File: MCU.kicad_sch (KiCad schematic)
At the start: 26 parts, among them J3 ST_LINK, SW1 Reset, U1 STM32G070CBT6, U5 LM4040DBZ-3, Y1 FC-135R_32.7680KA-AG0

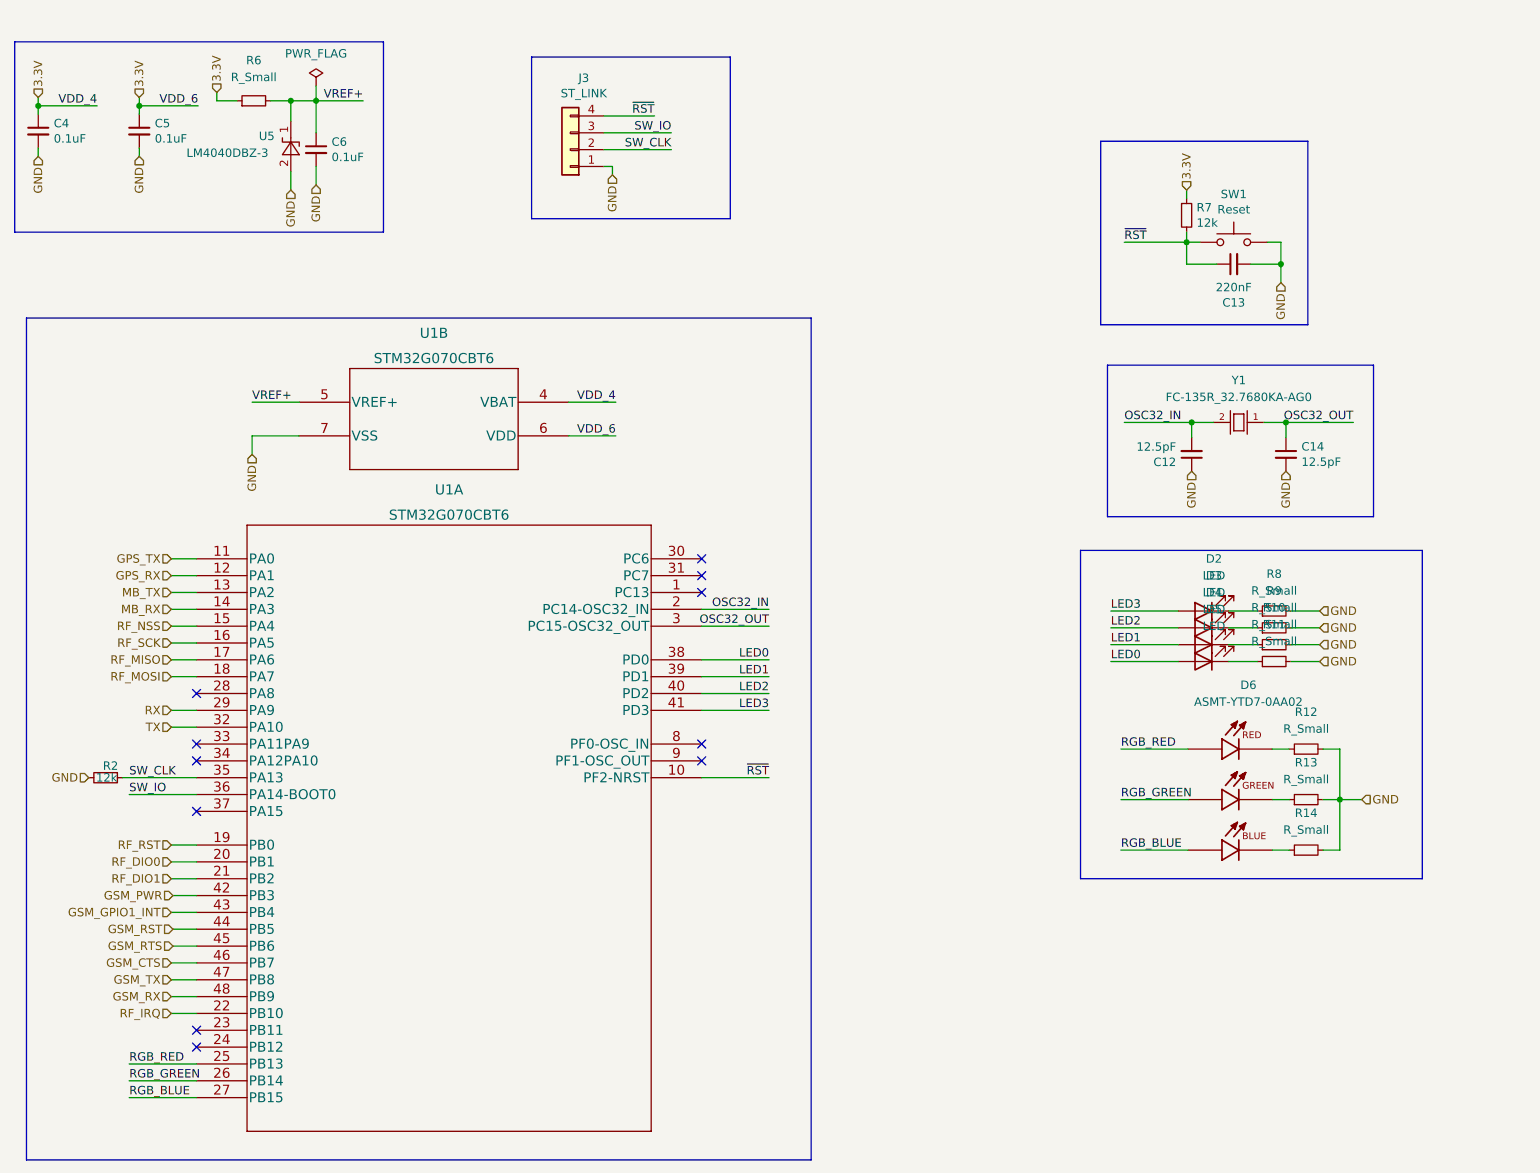
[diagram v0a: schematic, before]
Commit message: KiCad 0.2v
Schematics done.
Have to assign footprints to corresponding components.
Completely rework PCB.
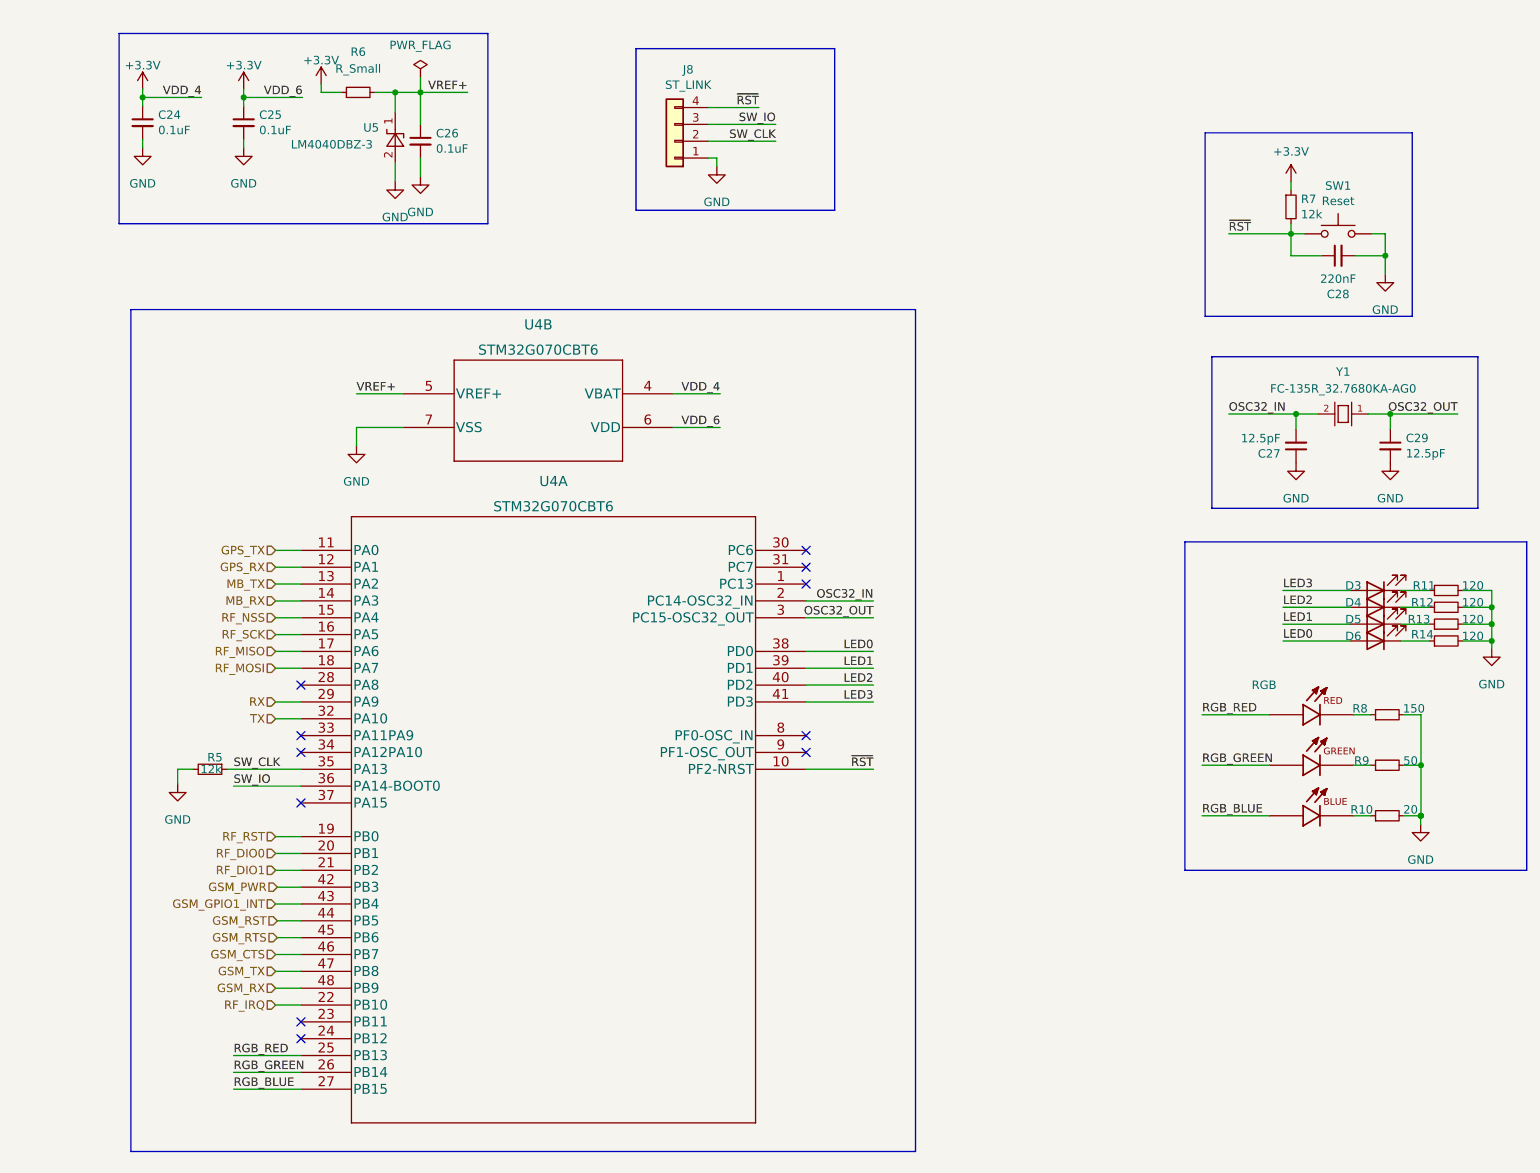
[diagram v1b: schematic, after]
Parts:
- removed C12, C14: 12.5pF, Capacitor_SMD:C_0603_1608Metric, symbol Device:C_Small
- removed C13: 220nF, Capacitor_SMD:C_0603_1608Metric, symbol Device:C_Small
- removed C4, C5, C6: 0.1uF, Capacitor_SMD:C_0603_1608Metric, symbol Device:C_Small
- removed D2: LED, symbol Device:LED
- removed D6: ASMT-YTD7-0AA02, LED_ASMT-YTD7-0AA02, symbol test:ASMT-YTD7-0AA02
- removed J3: ST_LINK, Connector_PinSocket_2.54mm:PinSocket_1x04_P2.54mm_Vertical, symbol Connector_Generic:Conn_01x04
- removed R2: 12k, Resistor_SMD:R_0603_1608Metric, symbol Device:R_Small
- removed U1: STM32G070CBT6, LQFP-48, symbol test:STM32G070CBT6
- added C24, C25, C26: 0.1uF, Capacitor_SMD:C_0603_1608Metric, symbol Device:C_Small
- added C27, C29: 12.5pF, Capacitor_SMD:C_0603_1608Metric, symbol Device:C_Small
- added C28: 220nF, Capacitor_SMD:C_0603_1608Metric, symbol Device:C_Small
- added D2: RGB, footprints:LED_ASMT-YTD7-0AA02, symbol test:ASMT-YTD7-0AA02
- added D6: LED, symbol Device:LED
- added J8: ST_LINK, Connector_PinSocket_2.54mm:PinSocket_1x04_P2.54mm_Vertical, symbol Connector_Generic:Conn_01x04
- added R5: 12k, Resistor_SMD:R_0603_1608Metric, symbol Device:R_Small
- added U4: STM32G070CBT6, LQFP-48, symbol test:STM32G070CBT6
- R10: value R_Small -> 20
- R11, R12, R13, R14: value R_Small -> 120
- R8: value R_Small -> 150
- R9: value R_Small -> 50
- Y1: footprint XTAL_FC-135R_32.7680KA-AG0 -> footprints:XTAL_FC-135R_32.7680KA-AG0
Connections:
- net GND: now also C24.2, C25.2, C26.2, C27.1, C28.2, C29.2, J8.1 (Pin_1), R5.2, U4.7 (VSS)
- net GPS_RX: now also U4.12 (PA1)
- net GPS_TX: now also U4.11 (PA0)
- net GSM_CTS: now also U4.46 (PB7)
- net GSM_GPIO1_INT: now also U4.43 (PB4)
- net GSM_PWR: now also U4.42 (PB3)
- net GSM_RST: now also U4.44 (PB5)
- net GSM_RTS: now also U4.45 (PB6)
- net GSM_RX: now also U4.48 (PB9)
- net GSM_TX: now also U4.47 (PB8)
- net LED0: now also D6.2 (A), U4.38 (PD0); no longer D5.2 (A)
- net LED1: now also D5.2 (A), U4.39 (PD1); no longer D4.2 (A)
- net LED2: now also D4.2 (A), U4.40 (PD2); no longer D3.2 (A)
- net LED3: now also D3.2 (A), U4.41 (PD3)
- net MB_RX: now also U4.14 (PA3)
- net MB_TX: now also U4.13 (PA2)
- net OSC32_IN: now also C27.2, U4.2 (PC14-OSC32_IN)
- net OSC32_OUT: now also C29.1, U4.3 (PC15-OSC32_OUT)
- net RF_DIO0: now also U4.20 (PB1)
- net RF_DIO1: now also U4.21 (PB2)
- net RF_IRQ: now also U4.22 (PB10)
- net RF_MISO: now also U4.17 (PA6)
- net RF_MOSI: now also U4.18 (PA7)
- net RF_NSS: now also U4.15 (PA4)
- net RF_RST: now also U4.19 (PB0)
- net RF_SCK: now also U4.16 (PA5)
- net RGB_BLUE: now also D2.6, U4.27 (PB15)
- net RGB_GREEN: now also D2.5, U4.26 (PB14)
- net RGB_RED: now also D2.4, U4.25 (PB13)
- net RX: now also U4.29 (PA9)
- net SW_CLK: now also J8.2 (Pin_2), R5.1, U4.35 (PA13)
- net SW_IO: now also J8.3 (Pin_3), U4.36 (PA14-BOOT0)
- net TX: now also U4.32 (PA10)
- net VREF+: now also C26.1, U4.5 (VREF+)
- net ~{RST}: now also C28.1, J8.4 (Pin_4), U4.10 (PF2-NRST)
- net at R13.1: now also D5.1 (K)
- net at R11.1: now also D3.1 (K); no longer D5.1 (K)
- net at R14.1: now also D6.1 (K)
- net at R9.1: now also D2.2; no longer D3.1 (K)
- net at R8.1: now also D2.3
- net at D4.1 (K): now also R12.1; no longer R10.1
- net 3.3V renamed +3V3
- net +3V3: now also C24.1, C25.1, U4.4 (VBAT), U4.6 (VDD)
- new net: D2.1, R10.1

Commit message: KiCad 0.3v
Improved aesthetics.
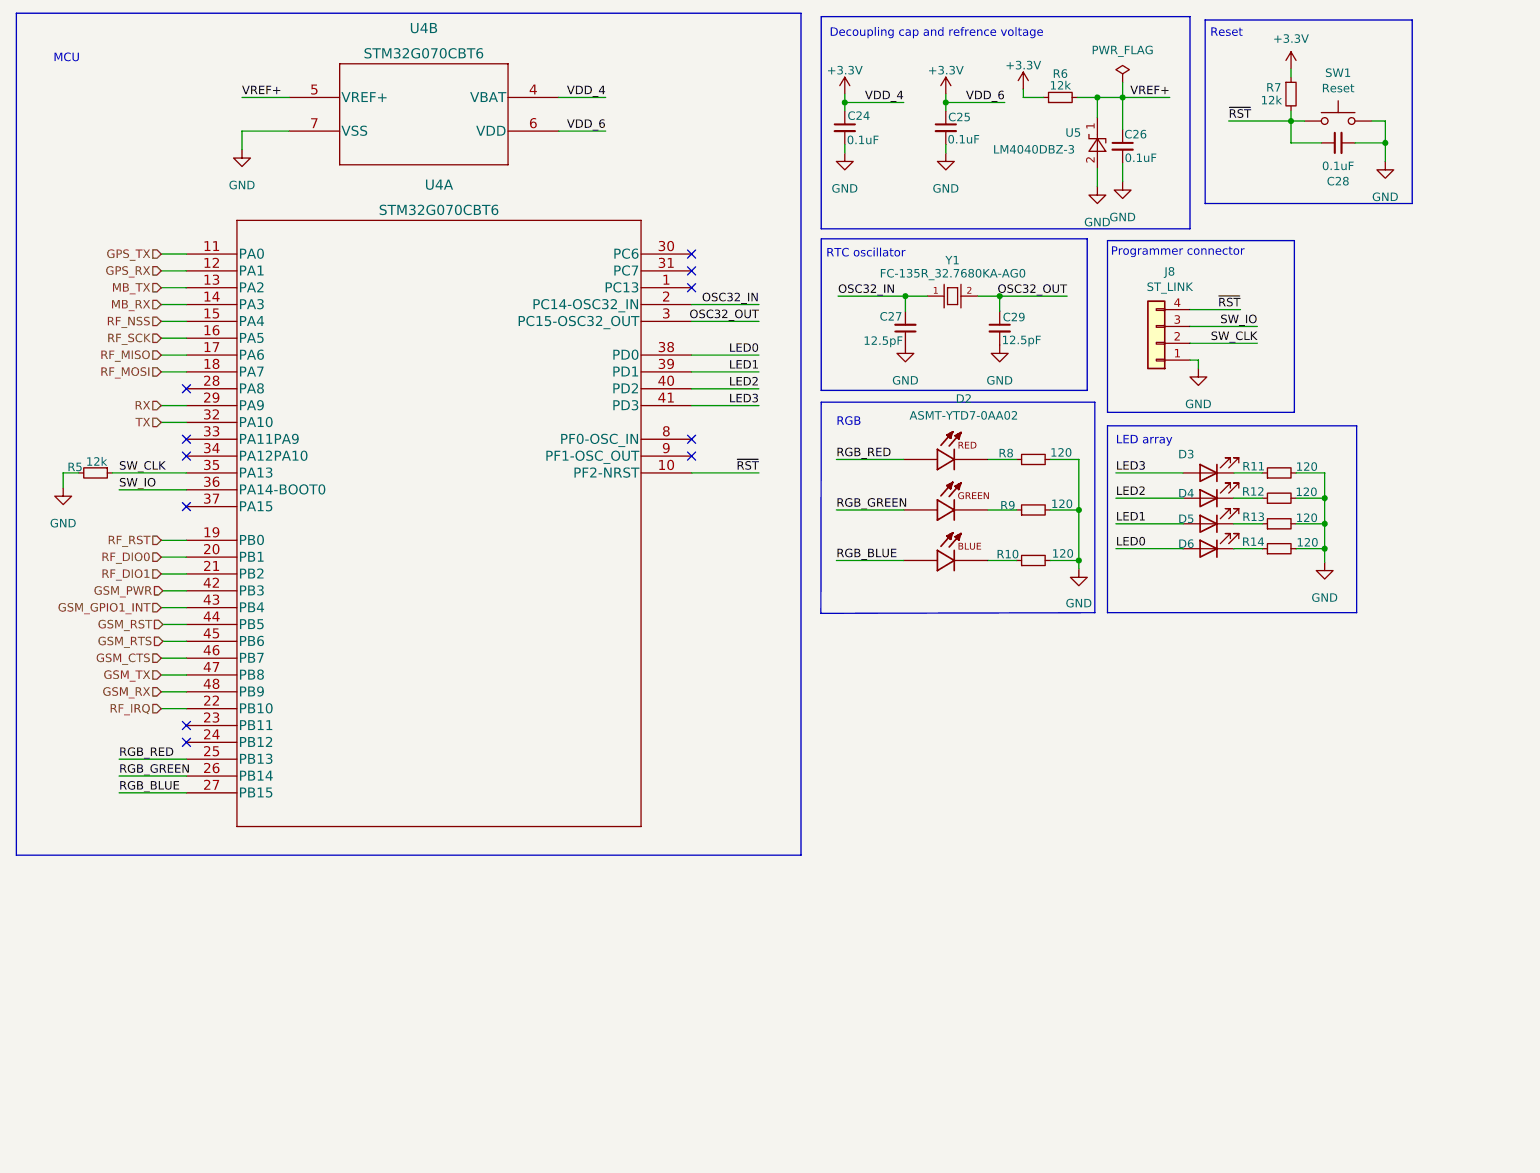
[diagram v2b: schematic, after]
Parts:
- removed D2: RGB, footprints:LED_ASMT-YTD7-0AA02, symbol test:ASMT-YTD7-0AA02
- removed Y1: FC-135R_32.7680KA-AG0, footprints:XTAL_FC-135R_32.7680KA-AG0, symbol test:FC-135R_32.7680KA-AG0
- added D2: ASMT-YTD7-0AA02, LED_ASMT-YTD7-0AA02, symbol schematics:ASMT-YTD7-0AA02
- added Y1: FC-135R_32.7680KA-AG0, XTAL_FC-135R_32.7680KA-AG0, symbol schematics:FC-135R_32.7680KA-AG0
- C28: value 220nF -> 0.1uF
- D3, D4, D5, D6: footprint (none) -> LED_SMD:LED_0603_1608Metric
- R10: value 20 -> 120; footprint (none) -> Resistor_SMD:R_0603_1608Metric
- R11, R12, R13, R14: footprint (none) -> Resistor_SMD:R_0603_1608Metric
- R6: value R_Small -> 12k; footprint (none) -> Resistor_SMD:R_0603_1608Metric
- R8: value 150 -> 120; footprint (none) -> Resistor_SMD:R_0603_1608Metric
- R9: value 50 -> 120; footprint (none) -> Resistor_SMD:R_0603_1608Metric
- U4: symbol test:STM32G070CBT6 -> schematics:STM32G070CBT6
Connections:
- net OSC32_IN: now also Y1.1
- net OSC32_OUT: now also Y1.2
- net RGB_BLUE: now also D2.6
- net RGB_GREEN: now also D2.5
- net RGB_RED: now also D2.4
- net at R9.1: now also D2.2
- net at R8.1: now also D2.3
- net at R10.1: now also D2.1
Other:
- note added: "Decoupling cap and refrence voltage"
- note added: "LED array"
- note added: "MCU"
- note added: "Programmer connector"
- note added: "RGB"
- note added: "RTC oscillator"
- note added: "Reset"
- moved on the sheet: C24, C25, C26, C27, C28, C29, D3, D4, D5, D6, J8, R10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

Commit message: 0.1v COM_PCB KiCad
First iteration of COM PCB.
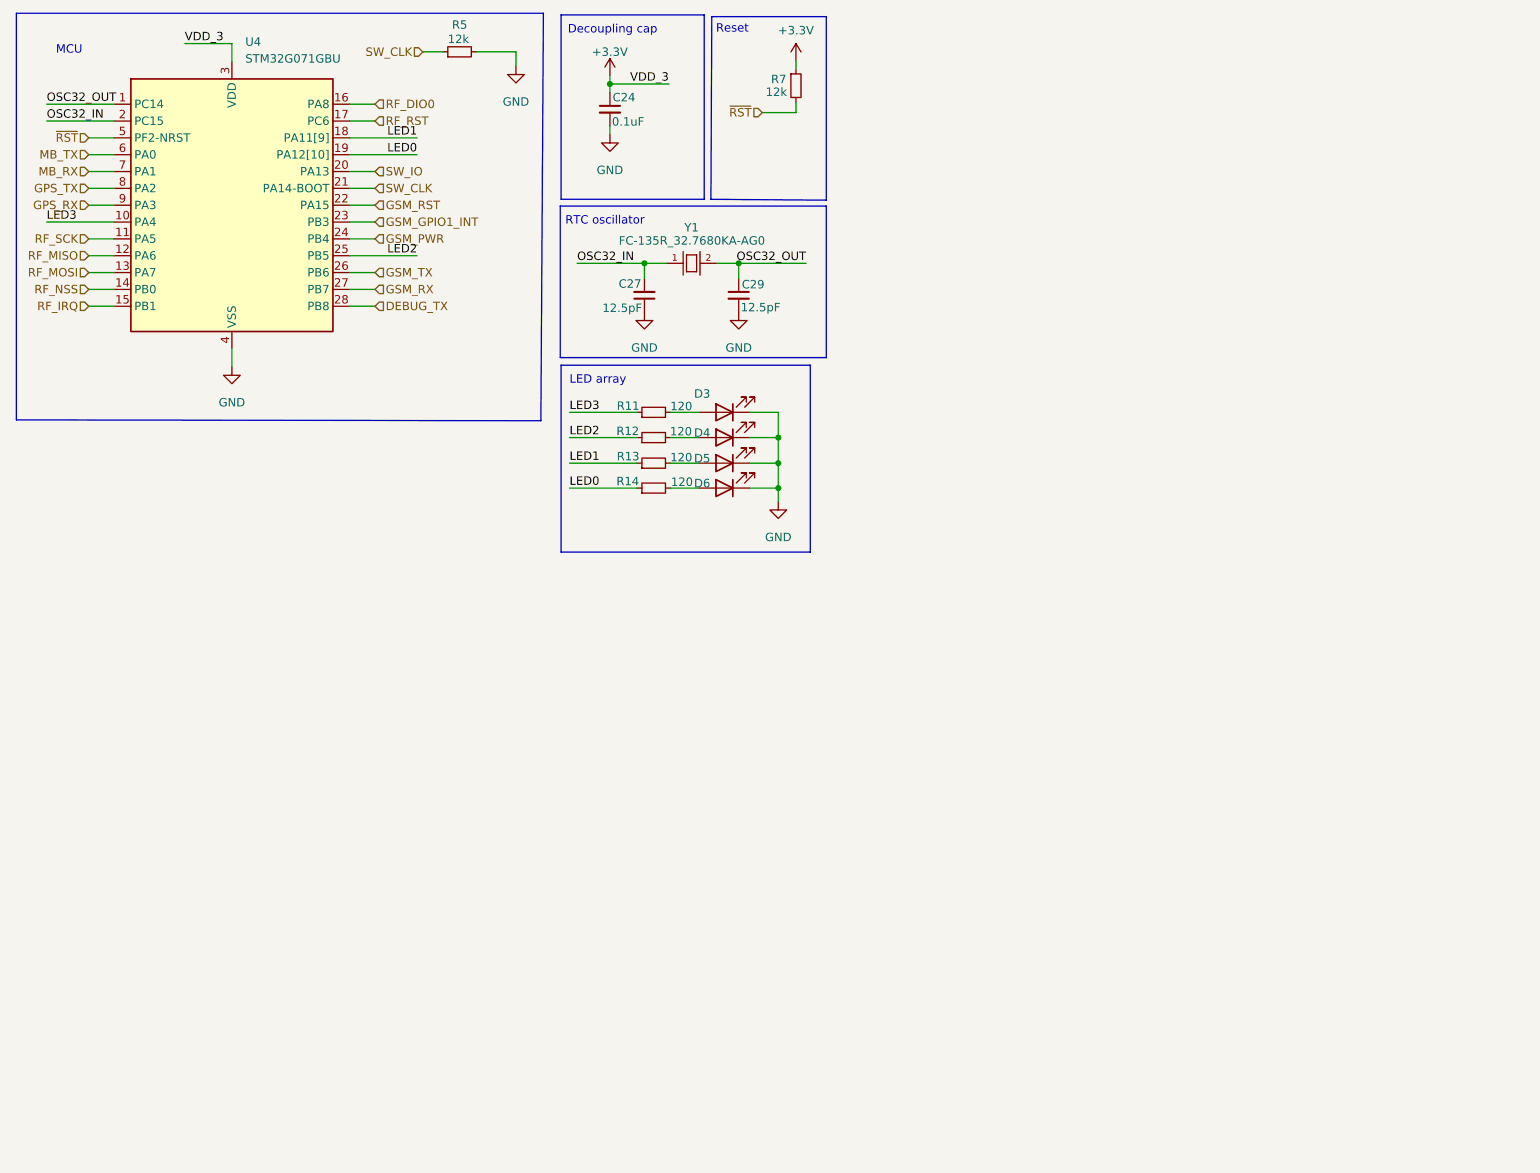
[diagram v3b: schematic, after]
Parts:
- removed C25, C26, C28: 0.1uF, Capacitor_SMD:C_0603_1608Metric, symbol Device:C_Small
- removed D2: ASMT-YTD7-0AA02, LED_ASMT-YTD7-0AA02, symbol schematics:ASMT-YTD7-0AA02
- removed J8: ST_LINK, Connector_PinSocket_2.54mm:PinSocket_1x04_P2.54mm_Vertical, symbol Connector_Generic:Conn_01x04
- removed R10, R8, R9: 120, Resistor_SMD:R_0603_1608Metric, symbol Device:R_Small
- removed R6: 12k, Resistor_SMD:R_0603_1608Metric, symbol Device:R_Small
- removed SW1: Reset, button:little_button, symbol Switch:SW_Push
- removed U4: STM32G070CBT6, LQFP-48, symbol schematics:STM32G070CBT6
- removed U5: LM4040DBZ-3, Package_TO_SOT_SMD:SOT-23, symbol Reference_Voltage:LM4040DBZ-3
- added U4: STM32G071GBU, Package_DFN_QFN:QFN-28_4x4mm_P0.5mm, symbol schematics:STM32G071GBU
- Y1: footprint XTAL_FC-135R_32.7680KA-AG0 -> footprints:XTAL_FC-135R_32.7680KA-AG0
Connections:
- net +3V3: now also U4.3 (VDD)
- net GND: now also D3.1 (K), D4.1 (K), D5.1 (K), D6.1 (K), U4.4 (VSS); no longer R11.2, R12.2, R13.2, R14.2
- net GPS_RX: now also U4.9 (PA3)
- net GPS_TX: now also U4.8 (PA2)
- net GSM_GPIO1_INT: now also U4.23 (PB3)
- net GSM_PWR: now also U4.24 (PB4)
- net GSM_RST: now also U4.22 (PA15)
- net GSM_RX: now also U4.27 (PB7)
- net GSM_TX: now also U4.26 (PB6)
- net LED0: now also R14.1, U4.19 (PA12[10]); no longer D6.2 (A)
- net LED1: now also R13.1, U4.18 (PA11[9]); no longer D5.2 (A)
- net LED2: now also R12.1, U4.25 (PB5); no longer D4.2 (A)
- net LED3: now also R11.1, U4.10 (PA4); no longer D3.2 (A)
- net MB_RX: now also U4.7 (PA1)
- net MB_TX: now also U4.6 (PA0)
- net OSC32_IN: now also U4.2 (PC15)
- net OSC32_OUT: now also U4.1 (PC14)
- net RF_DIO0: now also U4.16 (PA8)
- net RF_IRQ: now also U4.15 (PB1)
- net RF_MISO: now also U4.12 (PA6)
- net RF_MOSI: now also U4.13 (PA7)
- net RF_NSS: now also U4.14 (PB0)
- net RF_RST: now also U4.17 (PC6)
- net RF_SCK: now also U4.11 (PA5)
- net SW_CLK: now also U4.21 (PA14-BOOT)
- net SW_IO: now also U4.20 (PA13)
- net ~{RST}: now also U4.5 (PF2-NRST)
- new net: D4.2 (A), R12.2
- new net: D5.2 (A), R13.2
- new net: D6.2 (A), R14.2
- new net: D3.2 (A), R11.2
- new net DEBUG_TX: U4.28 (PB8)
- no-connect marks 11 -> 0
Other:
- note added: "Decoupling cap"
- note removed: "Decoupling cap and refrence voltage"
- note removed: "Programmer connector"
- note removed: "RGB"
- moved on the sheet: C24, C27, C29, D3, D4, D5, D6, R11, R12, R13, R14, R7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
